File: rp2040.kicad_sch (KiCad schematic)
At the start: 34 parts, among them Q3 AP2302B, SW1 SKPMAME010, SW2 SKPMAME010, SW3 SKPMAME010, SW4 SKPMAME010, SW5 SKPMAME010, SW6 SKPMAME010, U17 W25Q16JVUXIQ, U3 RP2040, Y2 12MHz

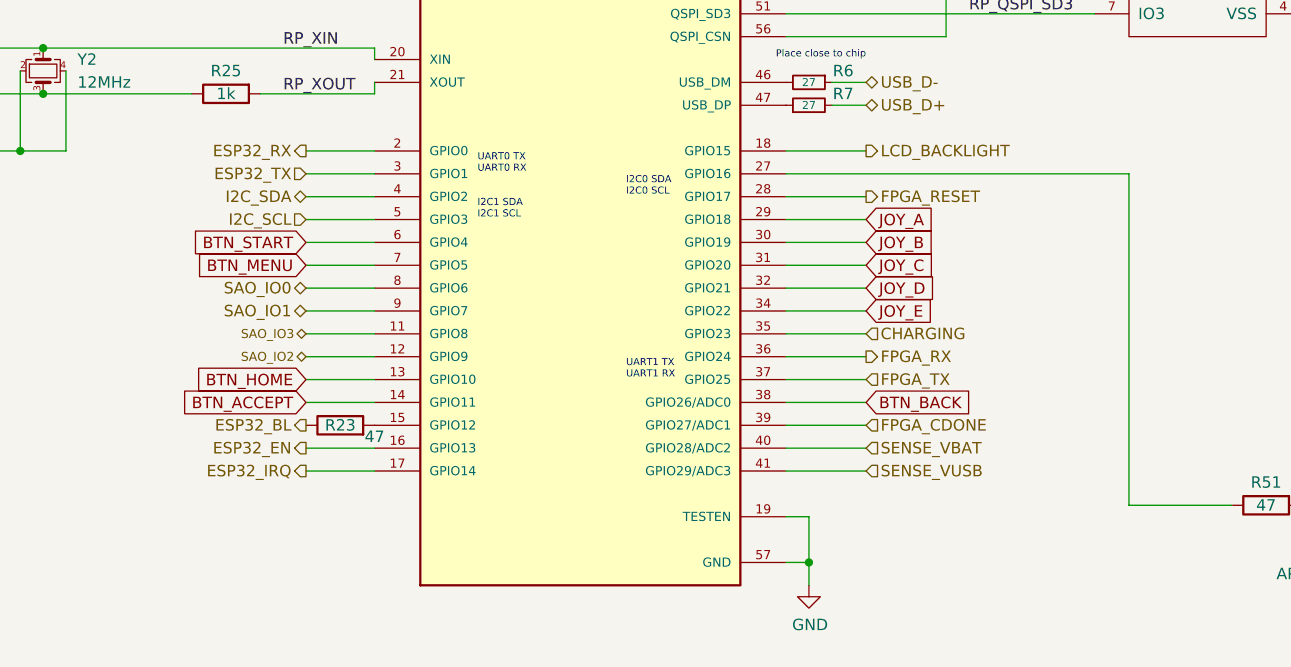
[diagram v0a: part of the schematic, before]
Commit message: Add lanyard holes, component placement
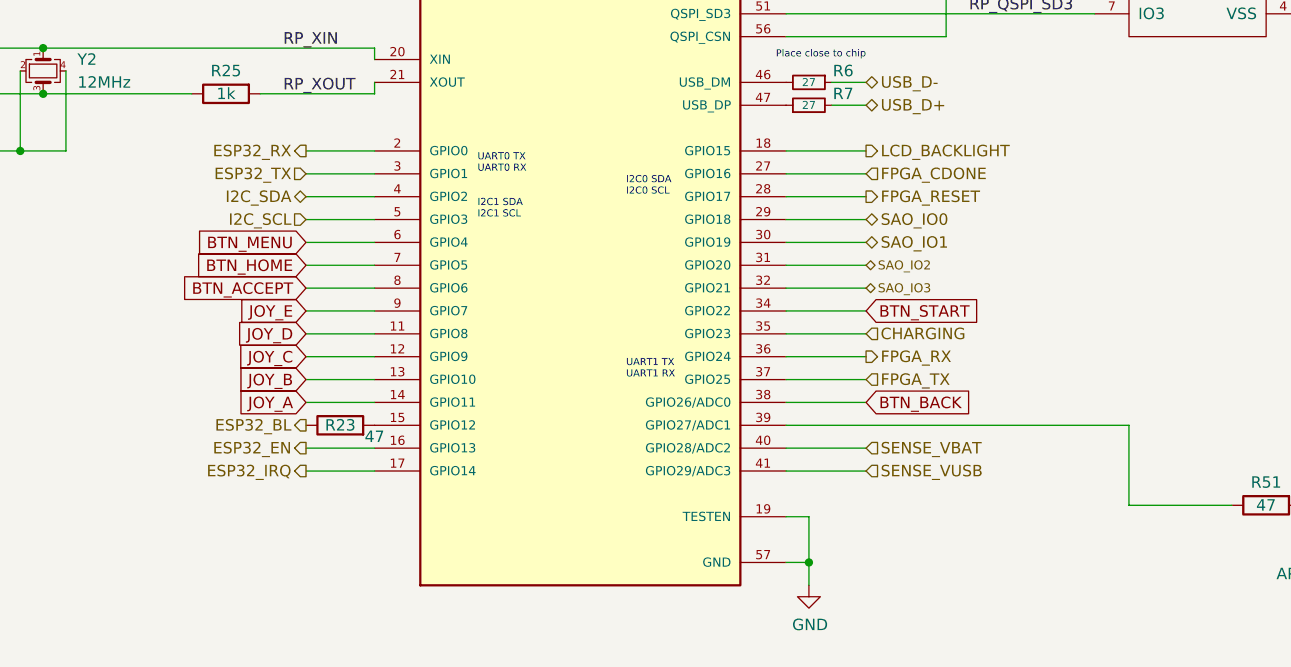
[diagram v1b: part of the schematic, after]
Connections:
- net BTN_ACCEPT: now also U3.8 (GPIO6); no longer U3.14 (GPIO11)
- net BTN_HOME: now also U3.7 (GPIO5); no longer U3.13 (GPIO10)
- net BTN_MENU: now also U3.6 (GPIO4); no longer U3.7 (GPIO5)
- net BTN_START: now also U3.34 (GPIO22); no longer U3.6 (GPIO4)
- net FPGA_CDONE: now also U3.27 (GPIO16); no longer U3.39 (GPIO27/ADC1)
- net JOY_A: now also U3.14 (GPIO11); no longer U3.29 (GPIO18)
- net JOY_B: now also U3.13 (GPIO10); no longer U3.30 (GPIO19)
- net JOY_C: now also U3.12 (GPIO9); no longer U3.31 (GPIO20)
- net JOY_D: now also U3.11 (GPIO8); no longer U3.32 (GPIO21)
- net JOY_E: now also U3.9 (GPIO7); no longer U3.34 (GPIO22)
- net SAO_IO0: now also U3.29 (GPIO18); no longer U3.8 (GPIO6)
- net SAO_IO1: now also U3.30 (GPIO19); no longer U3.9 (GPIO7)
- net SAO_IO2: now also U3.31 (GPIO20); no longer U3.12 (GPIO9)
- net SAO_IO3: now also U3.32 (GPIO21); no longer U3.11 (GPIO8)
- net at R51.1: now also U3.39 (GPIO27/ADC1); no longer U3.27 (GPIO16)
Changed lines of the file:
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@@
-    (stroke (width 0) (type default) (color 0 0 0 0))
-  )
-  (wire (pts (xy 193.04 95.25) (xy 154.94 95.25))
     (stroke (width 0) (type default) (color 0 0 0 0))
   )
@@
     (stroke (width 0) (type default) (color 0 0 0 0))
   )
+  (wire (pts (xy 193.04 123.19) (xy 193.04 132.08))
+    (stroke (width 0) (type default) (color 0 0 0 0))
+  )
   (wire (pts (xy 160.02 85.09) (xy 163.83 85.09))
     (stroke (width 0) (type default) (color 0 0 0 0))
@@
     (stroke (width 0) (type default) (color 0 0 0 0))
   )
-  (wire (pts (xy 154.94 123.19) (xy 163.83 123.19))
+  (wire (pts (xy 154.94 123.19) (xy 193.04 123.19))
     (stroke (width 0) (type default) (color 0 0 0 0))
   )
@@
     (stroke (width 0) (type default) (color 0 0 0 0))
   )
+  (wire (pts (xy 154.94 95.25) (xy 163.83 95.25))
+    (stroke (width 0) (type default) (color 0 0 0 0))
+  )
   (wire (pts (xy 191.77 50.8) (xy 191.77 53.34))
     (stroke (width 0) (type default) (color 0 0 0 0))
@@
   )
   (wire (pts (xy 154.94 62.23) (xy 165.1 62.23))
-    (stroke (width 0) (type default) (color 0 0 0 0))
-  )
-  (wire (pts (xy 193.04 95.25) (xy 193.04 132.08))
     (stroke (width 0) (type default) (color 0 0 0 0))
   )
@@
     )
   )
-  (global_label "JOY_D" (shape input) (at 163.83 107.95 0) (fields_autoplaced)
-    (effects (font (size 1.27 1.27)) (justify left))
-    (property "Intersheet References" "${INTERSHEET_REFS}" (id 0) (at 171.7785 107.8706 0)
-      (effects (font (size 1.27 1.27)) (justify left) hide)
-    )
-  )
-  (global_label "JOY_E" (shape input) (at 163.83 110.49 0) (fields_autoplaced)
-    (effects (font (size 1.27 1.27)) (justify left))
-    (property "Intersheet References" "${INTERSHEET_REFS}" (id 0) (at 171.6575 110.4106 0)
-      (effects (font (size 1.27 1.27)) (justify left) hide)
-    )
-  )
-  (global_label "BTN_HOME" (shape input) (at 101.6 118.11 180) (fields_autoplaced)
-    (effects (font (size 1.27 1.27)) (justify right))
-    (property "Intersheet References" "${INTERSHEET_REFS}" (id 0) (at 89.4787 118.1894 0)
-      (effects (font (size 1.27 1.27)) (justify right) hide)
-    )
-  )
-  (global_label "JOY_A" (shape input) (at 163.83 100.33 0) (fields_autoplaced)
-    (effects (font (size 1.27 1.27)) (justify left))
-    (property "Intersheet References" "${INTERSHEET_REFS}" (id 0) (at 269.24 234.95 0)
+  (global_label "JOY_D" (shape input) (at 101.6 113.03 180) (fields_autoplaced)
+    (effects (font (size 1.27 1.27)) (justify right))
+    (property "Intersheet References" "${INTERSHEET_REFS}" (id 0) (at 93.6515 113.1094 0)
+      (effects (font (size 1.27 1.27)) (justify right) hide)
+    )
+  )
+  (global_label "JOY_E" (shape input) (at 101.6 110.49 180) (fields_autoplaced)
+    (effects (font (size 1.27 1.27)) (justify right))
+    (property "Intersheet References" "${INTERSHEET_REFS}" (id 0) (at 93.7725 110.5694 0)
+      (effects (font (size 1.27 1.27)) (justify right) hide)
+    )
+  )
+  (global_label "BTN_HOME" (shape input) (at 101.6 105.41 180) (fields_autoplaced)
+    (effects (font (size 1.27 1.27)) (justify right))
+    (property "Intersheet References" "${INTERSHEET_REFS}" (id 0) (at 89.4787 105.4894 0)
+      (effects (font (size 1.27 1.27)) (justify right) hide)
+    )
+  )
+  (global_label "JOY_A" (shape input) (at 101.6 120.65 180) (fields_autoplaced)
+    (effects (font (size 1.27 1.27)) (justify right))
+    (property "Intersheet References" "${INTERSHEET_REFS}" (id 0) (at -3.81 -13.97 0)
       (effects (font (size 1.27 1.27)) hide)
     )
@@
     )
   )
-  (global_label "JOY_B" (shape input) (at 163.83 102.87 0) (fields_autoplaced)
-    (effects (font (size 1.27 1.27)) (justify left))
-    (property "Intersheet References" "${INTERSHEET_REFS}" (id 0) (at 171.7785 102.7906 0)
-      (effects (font (size 1.27 1.27)) (justify left) hide)
+  (global_label "JOY_B" (shape input) (at 101.6 118.11 180) (fields_autoplaced)
+    (effects (font (size 1.27 1.27)) (justify right))
+    (property "Intersheet References" "${INTERSHEET_REFS}" (id 0) (at 93.6515 118.1894 0)
+      (effects (font (size 1.27 1.27)) (justify right) hide)
     )
   )
@@
     )
   )
-  (global_label "BTN_START" (shape input) (at 101.6 102.87 180) (fields_autoplaced)
-    (effects (font (size 1.27 1.27)) (justify right))
-    (property "Intersheet References" "${INTERSHEET_REFS}" (id 0) (at 89.2368 102.7906 0)
-      (effects (font (size 1.27 1.27)) (justify right) hide)
-    )
-  )
-  (global_label "BTN_ACCEPT" (shape input) (at 101.6 120.65 180) (fields_autoplaced)
-    (effects (font (size 1.27 1.27)) (justify right))
-    (property "Intersheet References" "${INTERSHEET_REFS}" (id 0) (at 87.7248 120.5706 0)
-      (effects (font (size 1.27 1.27)) (justify right) hide)
-    )
-  )
-  (global_label "BTN_MENU" (shape input) (at 101.6 105.41 180) (fields_autoplaced)
-    (effects (font (size 1.27 1.27)) (justify right))
-    (property "Intersheet References" "${INTERSHEET_REFS}" (id 0) (at 89.4787 105.3306 0)
+  (global_label "BTN_START" (shape input) (at 163.83 110.49 0) (fields_autoplaced)
+    (effects (font (size 1.27 1.27)) (justify left))
+    (property "Intersheet References" "${INTERSHEET_REFS}" (id 0) (at 176.1932 110.5694 0)
+      (effects (font (size 1.27 1.27)) (justify left) hide)
+    )
+  )
+  (global_label "BTN_ACCEPT" (shape input) (at 101.6 107.95 180) (fields_autoplaced)
+    (effects (font (size 1.27 1.27)) (justify right))
+    (property "Intersheet References" "${INTERSHEET_REFS}" (id 0) (at 87.7248 107.8706 0)
+      (effects (font (size 1.27 1.27)) (justify right) hide)
+    )
+  )
+  (global_label "BTN_MENU" (shape input) (at 101.6 102.87 180) (fields_autoplaced)
+    (effects (font (size 1.27 1.27)) (justify right))
+    (property "Intersheet References" "${INTERSHEET_REFS}" (id 0) (at 89.4787 102.7906 0)
       (effects (font (size 1.27 1.27)) (justify right) hide)
     )
@@
     )
   )
-  (global_label "JOY_C" (shape input) (at 163.83 105.41 0) (fields_autoplaced)
-    (effects (font (size 1.27 1.27)) (justify left))
-    (property "Intersheet References" "${INTERSHEET_REFS}" (id 0) (at 171.7785 105.3306 0)
-      (effects (font (size 1.27 1.27)) (justify left) hide)
+  (global_label "JOY_C" (shape input) (at 101.6 115.57 180) (fields_autoplaced)
+    (effects (font (size 1.27 1.27)) (justify right))
+    (property "Intersheet References" "${INTERSHEET_REFS}" (id 0) (at 93.6515 115.6494 0)
+      (effects (font (size 1.27 1.27)) (justify right) hide)
     )
   )
@@
     (effects (font (size 1.27 1.27)) (justify left))
   )
-  (hierarchical_label "SAO_IO3" (shape bidirectional) (at 101.6 113.03 180)
-    (effects (font (size 1 1)) (justify right))
-  )
-  (hierarchical_label "SAO_IO1" (shape bidirectional) (at 101.6 110.49 180)
-    (effects (font (size 1.27 1.27)) (justify right))
+  (hierarchical_label "SAO_IO3" (shape bidirectional) (at 163.83 107.95 0)
+    (effects (font (size 1 1)) (justify left))
+  )
+  (hierarchical_label "SAO_IO1" (shape bidirectional) (at 163.83 102.87 0)
+    (effects (font (size 1.27 1.27)) (justify left))
   )
   (hierarchical_label "ESP32_RX" (shape output) (at 101.6 92.71 180)
@@
     (effects (font (size 1.27 1.27)) (justify left))
   )
-  (hierarchical_label "SAO_IO2" (shape bidirectional) (at 101.6 115.57 180)
-    (effects (font (size 1 1)) (justify right))
+  (hierarchical_label "SAO_IO2" (shape bidirectional) (at 163.83 105.41 0)
+    (effects (font (size 1 1)) (justify left))
   )
   (hierarchical_label "FPGA_TX" (shape input) (at 163.83 118.11 0)
@@
     (effects (font (size 1.27 1.27)) (justify left))
   )
-  (hierarchical_label "FPGA_CDONE" (shape input) (at 163.83 123.19 0)
+  (hierarchical_label "FPGA_CDONE" (shape input) (at 163.83 95.25 0)
     (effects (font (size 1.27 1.27)) (justify left))
   )
@@
     (effects (font (size 1.27 1.27)) (justify left))
   )
-  (hierarchical_label "SAO_IO0" (shape bidirectional) (at 101.6 107.95 180)
-    (effects (font (size 1.27 1.27)) (justify right))
+  (hierarchical_label "SAO_IO0" (shape bidirectional) (at 163.83 100.33 0)
+    (effects (font (size 1.27 1.27)) (justify left))
   )
   (symbol (lib_id "mch2021-rescue:C-Device") (at 137.16 167.64 0) (unit 1)

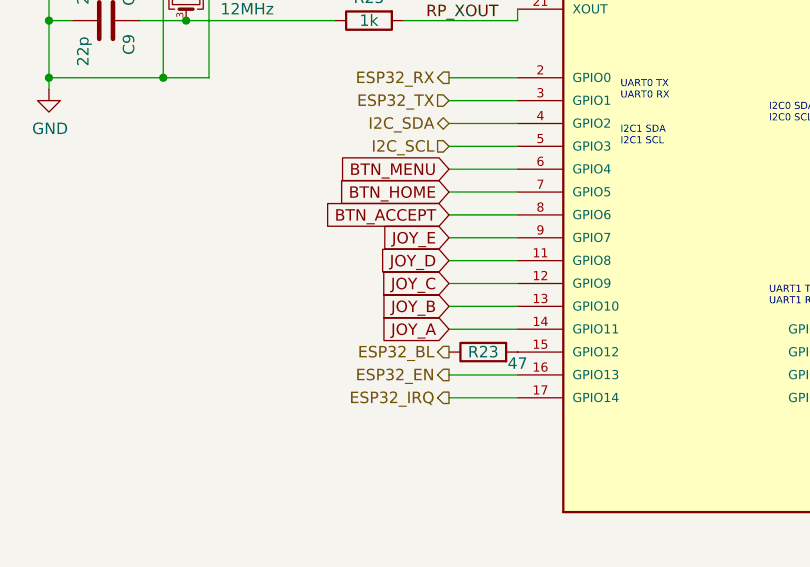
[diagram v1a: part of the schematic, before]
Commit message: Got some of the routing done
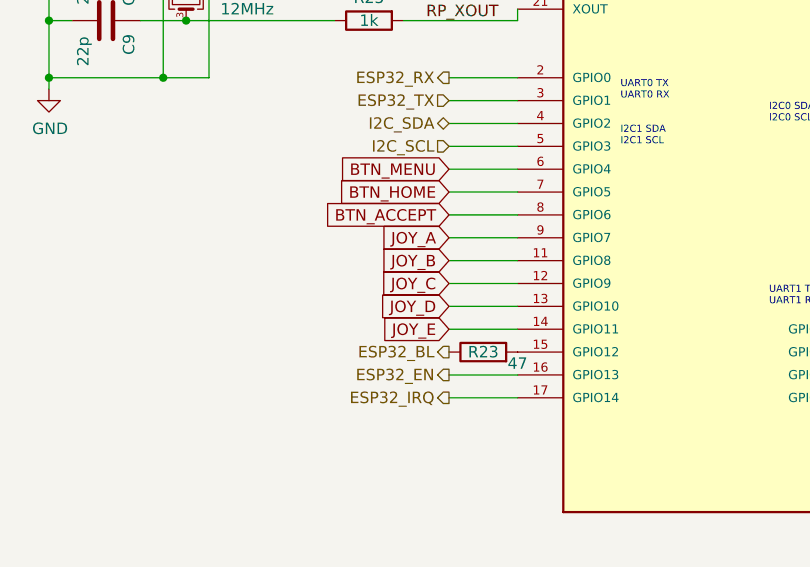
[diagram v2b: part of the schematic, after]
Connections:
- net JOY_A: now also U3.9 (GPIO7); no longer U3.14 (GPIO11)
- net JOY_B: now also U3.11 (GPIO8); no longer U3.13 (GPIO10)
- net JOY_D: now also U3.13 (GPIO10); no longer U3.11 (GPIO8)
- net JOY_E: now also U3.14 (GPIO11); no longer U3.9 (GPIO7)
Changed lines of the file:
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@@
     )
   )
-  (global_label "JOY_D" (shape input) (at 101.6 113.03 180) (fields_autoplaced)
+  (global_label "JOY_D" (shape input) (at 101.6 118.11 180) (fields_autoplaced)
     (effects (font (size 1.27 1.27)) (justify right))
-    (property "Intersheet References" "${INTERSHEET_REFS}" (id 0) (at 93.6515 113.1094 0)
+    (property "Intersheet References" "${INTERSHEET_REFS}" (id 0) (at 93.6515 118.1894 0)
       (effects (font (size 1.27 1.27)) (justify right) hide)
     )
   )
-  (global_label "JOY_E" (shape input) (at 101.6 110.49 180) (fields_autoplaced)
+  (global_label "JOY_E" (shape input) (at 101.6 120.65 180) (fields_autoplaced)
     (effects (font (size 1.27 1.27)) (justify right))
-    (property "Intersheet References" "${INTERSHEET_REFS}" (id 0) (at 93.7725 110.5694 0)
+    (property "Intersheet References" "${INTERSHEET_REFS}" (id 0) (at 93.7725 120.7294 0)
       (effects (font (size 1.27 1.27)) (justify right) hide)
     )
@@
     )
   )
-  (global_label "JOY_A" (shape input) (at 101.6 120.65 180) (fields_autoplaced)
+  (global_label "JOY_A" (shape input) (at 101.6 110.49 180) (fields_autoplaced)
     (effects (font (size 1.27 1.27)) (justify right))
-    (property "Intersheet References" "${INTERSHEET_REFS}" (id 0) (at -3.81 -13.97 0)
+    (property "Intersheet References" "${INTERSHEET_REFS}" (id 0) (at -3.81 -24.13 0)
       (effects (font (size 1.27 1.27)) hide)
     )
@@
     )
   )
-  (global_label "JOY_B" (shape input) (at 101.6 118.11 180) (fields_autoplaced)
+  (global_label "JOY_B" (shape input) (at 101.6 113.03 180) (fields_autoplaced)
     (effects (font (size 1.27 1.27)) (justify right))
-    (property "Intersheet References" "${INTERSHEET_REFS}" (id 0) (at 93.6515 118.1894 0)
+    (property "Intersheet References" "${INTERSHEET_REFS}" (id 0) (at 93.6515 113.1094 0)
       (effects (font (size 1.27 1.27)) (justify right) hide)
     )
